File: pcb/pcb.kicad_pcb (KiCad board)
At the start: 2 copper layers, 137.5 x 93.4 mm, 51 parts, among them SW1 SW_SPST, SW10 SW_SPST, SW11 SW_SPST, SW12 SW_SPST, SW13 SW_SPST, SW14 SW_SPST, SW15 SW_SPST, SW16 SW_SPST, SW17 SW_SPST, SW18 SW_SPST, SW19 SW_SPST, SW2 SW_SPST, SW20 SW_SPST, SW21 SW_SPST, SW3 SW_SPST, SW4 SW_SPST, SW5 SW_SPST, SW6 SW_SPST, SW7 SW_SPST, SW8 SW_SPST, SW9 SW_SPST, U1 XIAO_nRF52840

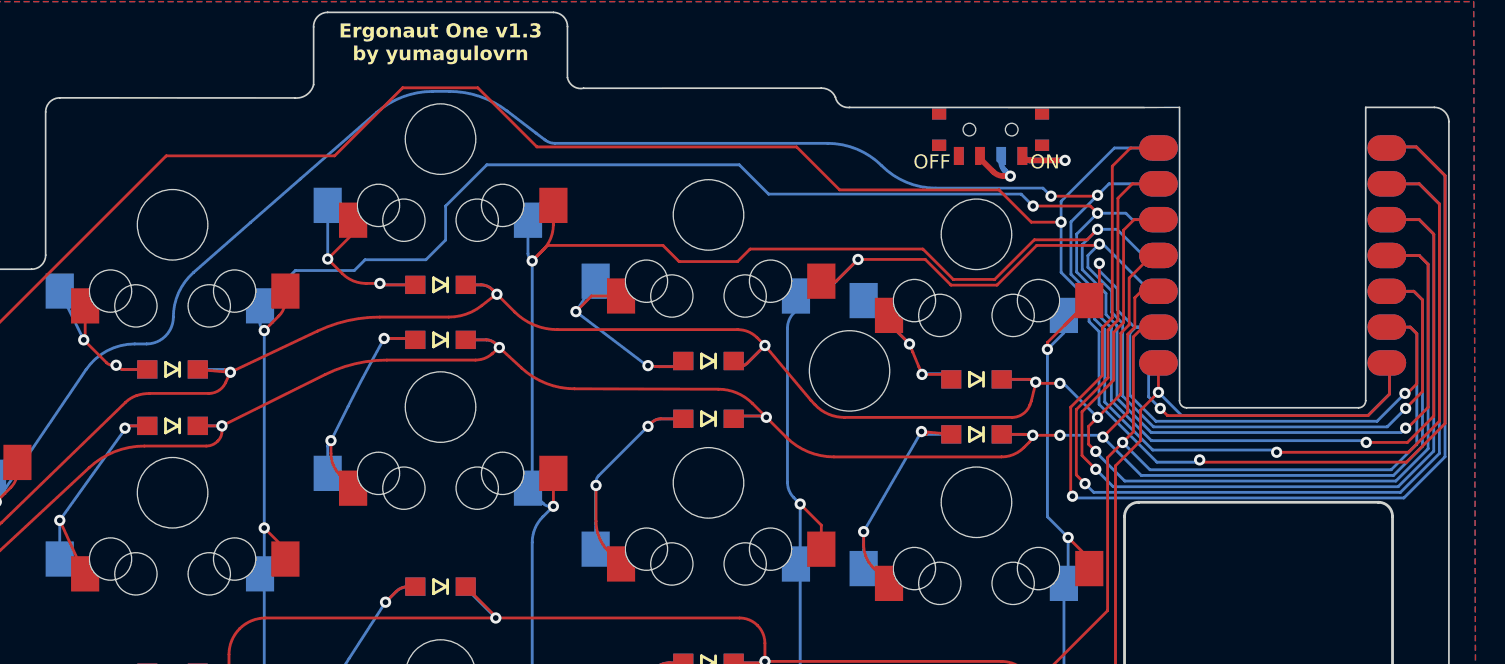
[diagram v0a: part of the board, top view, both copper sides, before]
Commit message: красоту навёл
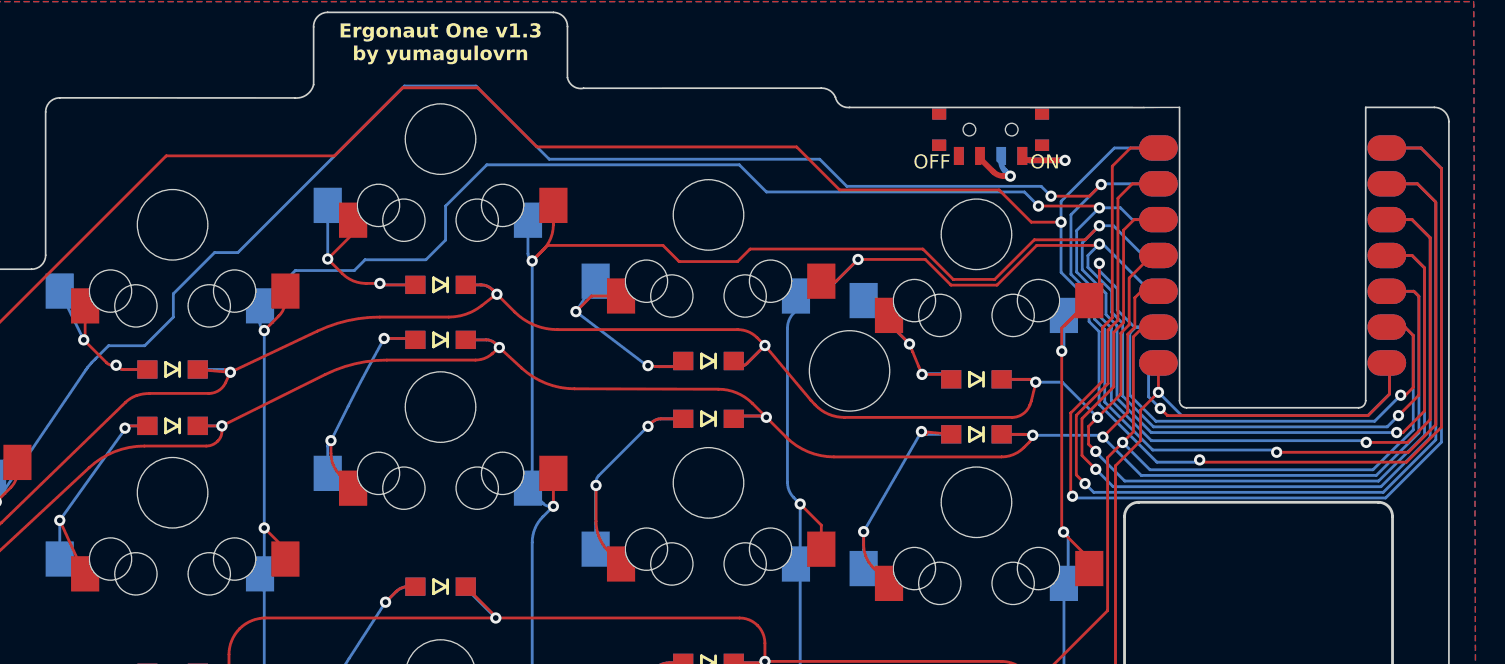
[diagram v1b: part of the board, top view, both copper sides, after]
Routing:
- net C1: track 202.8 -> 205.6 mm
- net unconnected-(U1-3V3-Pad12)_1: track 65.1 -> 63.9 mm
- net R2: track 198.3 -> 197.1 mm
- net R0: track 200.6 -> 199.5 mm, vias 9 -> 8
- net C5: track 142.1 -> 141.0 mm
- net GND: track 72.6 -> 71.6 mm
- net R1: track 185.5 -> 184.6 mm, vias 8 -> 7
- net unconnected-(U1-5V-Pad14): track 80.2 -> 79.3 mm

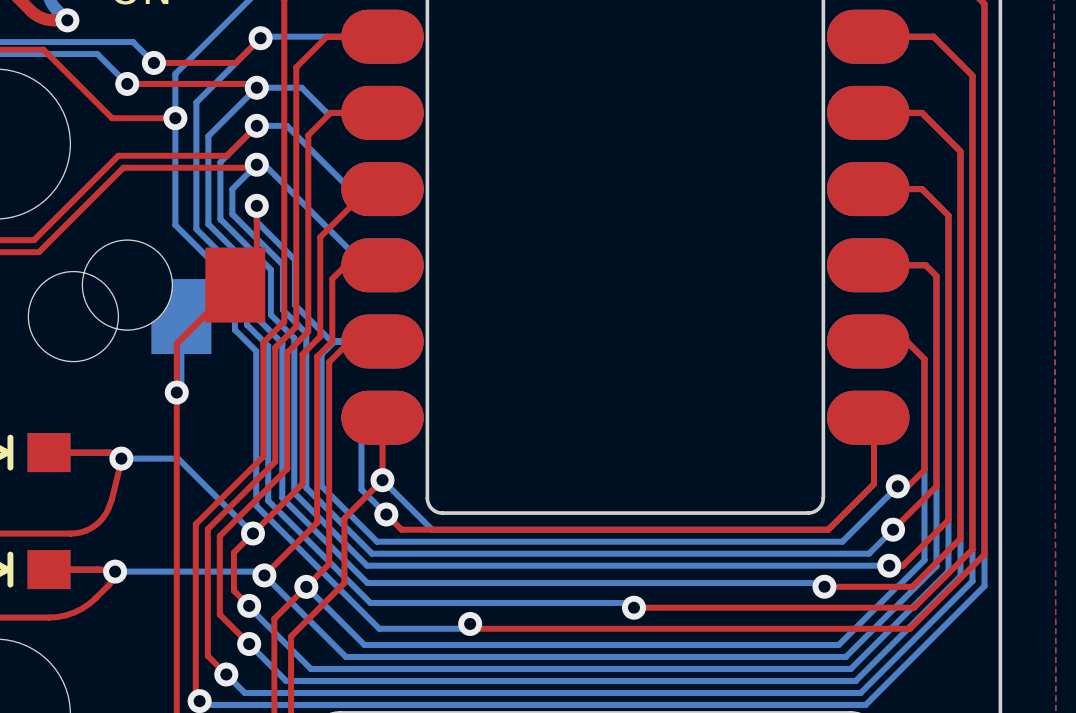
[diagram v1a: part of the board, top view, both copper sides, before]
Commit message: Выровнял по Z
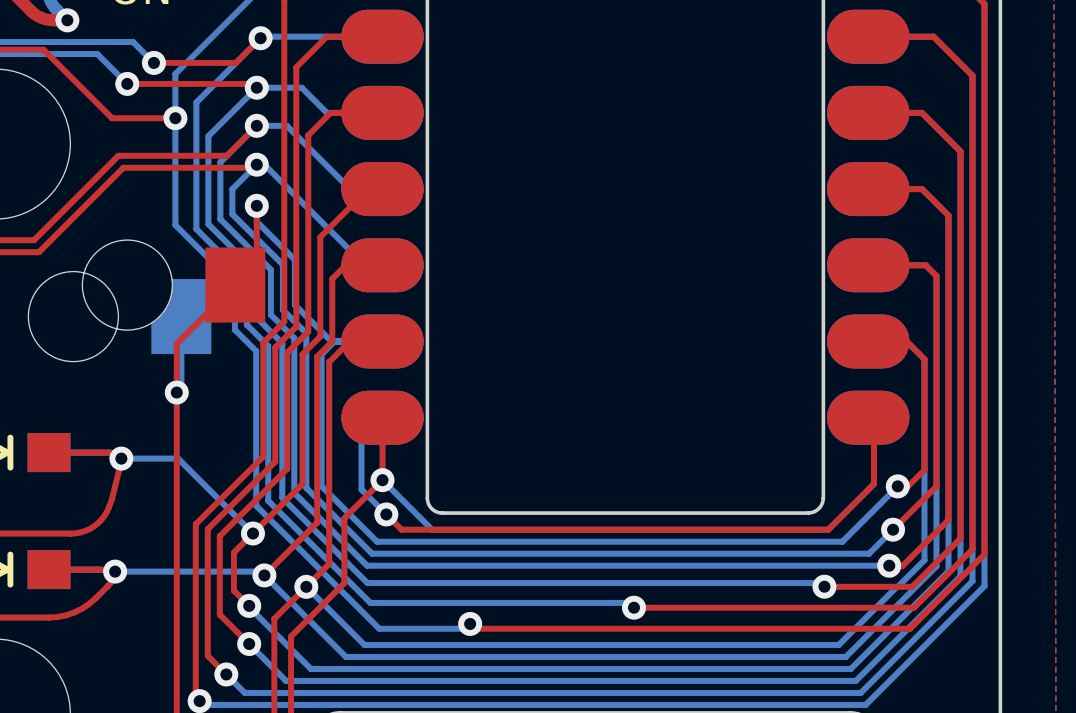
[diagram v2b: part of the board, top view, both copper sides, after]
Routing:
- net C5: track 141.0 -> 136.8 mm
- net R2: track 197.1 -> 195.9 mm
- net R3: track 129.6 -> 128.5 mm
- net C4: track 154.3 -> 153.4 mm
- net C3: track 176.5 -> 175.6 mm
- net unconnected-(U1-B8_TX/1.11-Pad7)_1: track 23.2 -> 22.4 mm
- net R1: track 184.6 -> 183.9 mm
